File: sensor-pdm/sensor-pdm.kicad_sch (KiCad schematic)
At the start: 27 parts, among them J1 43045-0600, J2 43045-0800, J3 43045-1200

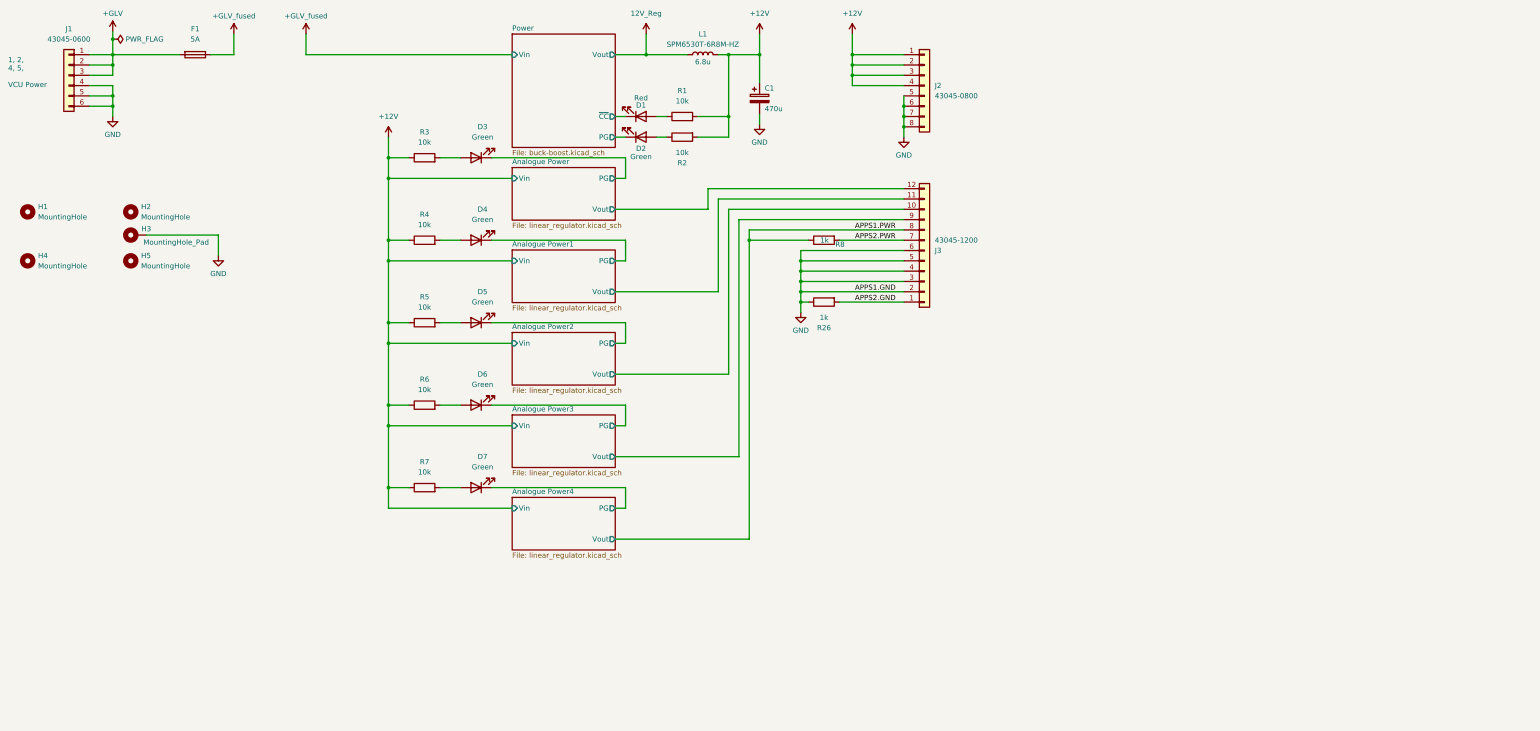
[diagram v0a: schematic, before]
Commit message: pcb basically done, needs a bit of silkscreen
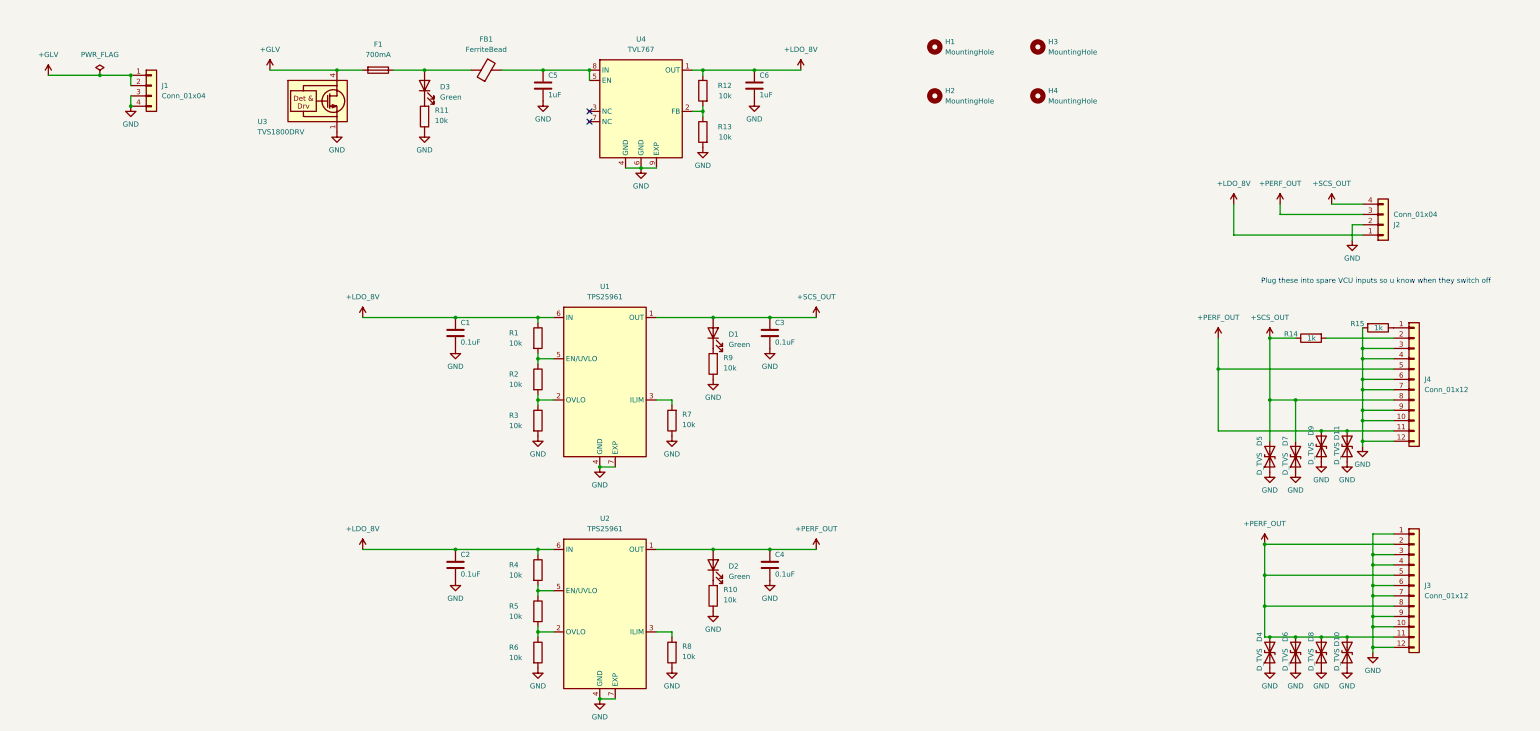
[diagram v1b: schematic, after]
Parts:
- removed C1: 470u, Capacitor_THT:CP_Radial_D10.0mm_P5.00mm, symbol Device:C_Polarized
- removed D4, D5, D6, D7: Green, LED_SMD:LED_0603_1608Metric, symbol Device:LED
- removed H3: MountingHole_Pad, MountingHole:MountingHole_3.2mm_M3_Pad_Via, symbol Mechanical:MountingHole_Pad
- removed J1: 43045-0600, Connector_Molex:Molex_Micro-Fit_3.0_43045-0600_2x03_P3.00mm_Horizontal, symbol Connector_Generic:Conn_01x06
- removed J2: 43045-0800, Connector_Molex:Molex_Micro-Fit_3.0_43045-0800_2x04_P3.00mm_Horizontal, symbol Connector_Generic:Conn_01x08
- removed L1: 6.8u, SamacSys:SPM6530, symbol Device:L
- removed R26: 1k, Resistor_SMD:R_0603_1608Metric, symbol Device:R
- added C1, C2, C3, C4: 0.1uF, Capacitor_SMD:C_0603_1608Metric_Pad1.08x0.95mm_HandSolder, symbol Device:C
- added C5, C6: 1uF, Capacitor_SMD:C_0603_1608Metric_Pad1.08x0.95mm_HandSolder, symbol Device:C
- added D10, D11, D4, D5, D6, D7, D8, D9: D_TVS, SUFST:D_SOD-323_wide, symbol Device:D_TVS
- added FB1: FerriteBead, Inductor_SMD:L_0805_2012Metric_Pad1.05x1.20mm_HandSolder, symbol Device:FerriteBead
- added J1, J2: Conn_01x04, Connector_Molex:Molex_Micro-Fit_3.0_43045-0400_2x02_P3.00mm_Horizontal, symbol Connector_Generic:Conn_01x04
- added J4: Conn_01x12, Molex_Micro-Fit_3.0_43045-1200_2x06_P3.00mm_Horizontal, symbol Connector_Generic:Conn_01x12
- added R10, R11, R12, R13, R9: 10k, Resistor_SMD:R_0603_1608Metric_Pad0.98x0.95mm_HandSolder, symbol Device:R
- added R14, R15: 1k, Resistor_SMD:R_0603_1608Metric_Pad0.98x0.95mm_HandSolder, symbol Device:R
- added U1, U2: TPS25961, SUFST:TPS73733DRVR, symbol SUFST:TPS25961
- added U3: TVS1800DRV, Package_SON:WSON-6-1EP_2x2mm_P0.65mm_EP1x1.6mm, symbol Power_Protection:TVS1800DRV
- added U4: TVL767, Package_SO:HVSSOP-8-1EP_3x3mm_P0.65mm_EP1.57x1.89mm, symbol SUFST:TLV767
- D1: value Red -> Green; footprint LED_SMD:LED_0603_1608Metric -> LED_SMD:LED_0603_1608Metric_Pad1.05x0.95mm_HandSolder; Mouser Part Number 755-SML-D12U1WT86 -> 755-SML-D12P8WT86
- D2, D3: footprint LED_SMD:LED_0603_1608Metric -> LED_SMD:LED_0603_1608Metric_Pad1.05x0.95mm_HandSolder
- F1: value 5A -> 700mA; footprint Fuse:Fuse_0603_1608Metric -> Fuse:Fuse_0603_1608Metric_Pad1.05x0.95mm_HandSolder
- J3: value 43045-1200 -> Conn_01x12; footprint Connector_Molex:Molex_Micro-Fit_3.0_43045-1200_2x06_P3.00mm_Horizontal -> Molex_Micro-Fit_3.0_43045-1200_2x06_P3.00mm_Horizontal; To Order INV -> (none)
- R1, R2, R3, R4, R5, R6, R7: footprint Resistor_SMD:R_0603_1608Metric -> Resistor_SMD:R_0603_1608Metric_Pad0.98x0.95mm_HandSolder
- R8: value 1k -> 10k; footprint Resistor_SMD:R_0603_1608Metric -> Resistor_SMD:R_0603_1608Metric_Pad0.98x0.95mm_HandSolder
- renumbered H4 to H2, H2 to H3, H5 to H4
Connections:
- net +GLV_fused is gone; now on an unnamed net: F1.1
- net APPS2.GND is gone; now on net GND: J3.1 (Pin_1)
- net Analogue Power/Vout is gone; now on net GND: J3.12 (Pin_12)
- net Analogue Power1/Vout is gone; now on net +PERF_OUT: J3.11 (Pin_11)
- net Analogue Power2/Vout is gone; now on net GND: J3.10 (Pin_10)
- net Analogue Power3/Vout is gone; now on net GND: J3.9 (Pin_9)
- net +GLV: now also J1.1 (Pin_1), J1.2 (Pin_2), U3.4 (IN), U3.5 (IN), U3.6 (IN)
- net GND: now also J3.7 (Pin_7), R3.2, R6.2, R7.1, R8.1, C1.1, C2.1, C3.1, C4.1, C5.1, C6.1, D10.1 (A1), D11.1 (A1), D4.1 (A1), D5.1 (A1), D6.1 (A1), D7.1 (A1), D8.1 (A1), D9.1 (A1), J1.3 (Pin_3), J1.4 (Pin_4), J2.2 (Pin_2), J4.10 (Pin_10), J4.12 (Pin_12), J4.3 (Pin_3), J4.4 (Pin_4), J4.6 (Pin_6), J4.7 (Pin_7), J4.9 (Pin_9), R10.1, R11.1, R13.2, R15.2, R9.1, U1.4 (GND), U1.7 (EXP), U2.4 (GND), U2.7 (EXP), U3.1 (GND), U3.2 (GND), U3.3 (GND), U3.7 (GND), U4.4 (GND), U4.6 (GND), U4.9 (EXP); no longer J3.2 (Pin_2), J3.5 (Pin_5)
- net at D3.2 (A): now also FB1.1; no longer R3.2
- net at R7.2: now also U1.3 (ILIM)
- net +LDO_8V: now reaches R1.1
- net +LDO_8V: now also R4.1, C1.2, C2.2, C6.2, J2.1 (Pin_1), R12.1, U1.6 (IN), U2.6 (IN), U4.1 (OUT); no longer D1.2 (A)
- net at R4.2: now also R5.1, U2.5 (EN/UVLO)
- net at R2.1: now also R1.2, U1.5 (EN/UVLO); no longer D2.2 (A)
- net at R5.2: now also R6.1, U2.2 (OVLO)
- removed net +12V: R1.2, R2.2, R3.1, R4.1, R5.1, R6.1, R7.1
- net APPS1.PWR renamed +PERF_OUT
- net +PERF_OUT: now also D2.2 (A), J3.2 (Pin_2), J3.5 (Pin_5), C4.2, D10.2 (A2), D11.2 (A2), D4.2 (A2), D6.2 (A2), D8.2 (A2), D9.2 (A2), J2.3 (Pin_3), J4.11 (Pin_11), J4.5 (Pin_5), U2.1 (OUT); no longer R8.1
- net APPS2.PWR: no longer names the net of R8.2
- net APPS2.PWR: now also U2.3 (ILIM); no longer J3.7 (Pin_7)
- net Analogue Power/PG: no longer names the net of D3.1 (K)
- net Analogue Power/PG: now also R11.2
- net Power/PG: no longer names the net of D2.1 (K)
- net Power/PG: now also R10.2
- net Power/~{CC}: no longer names the net of D1.1 (K)
- net Power/~{CC}: now also R9.2
- new net: J4.1 (Pin_1), R15.1
- new net: R12.2, R13.1, U4.2 (FB)
- new net: R2.2, R3.1, U1.2 (OVLO)
- new net: J4.2 (Pin_2), R14.2
- new net: C5.2, FB1.2, U4.5 (EN), U4.8 (IN)
- new net +SCS_OUT: C3.2, D1.2 (A), D5.2 (A2), D7.2 (A2), J2.4 (Pin_4), J4.8 (Pin_8), R14.1, U1.1 (OUT)
- no-connect marks 0 -> 2
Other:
- removed sheet Analogue Power
- removed sheet Analogue Power1
- removed sheet Analogue Power2
- removed sheet Analogue Power3
- removed sheet Analogue Power4
- removed sheet Power
- note added: "Plug these into spare VCU inputs so u know when they switch off"
- note removed: "1, 2, 4, 5, VCU Power"
- moved on the sheet: H1, H2, H3, H4
